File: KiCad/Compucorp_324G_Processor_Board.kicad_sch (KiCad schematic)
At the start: 9 parts, among them J5 Processor Interboard, J6 Unused Connector, U5 TMC1872 (TCL07), U6 TMC1866 (TCL06), U7 TMC1867 (TCL05), U8 TMC1870 (TCL04)

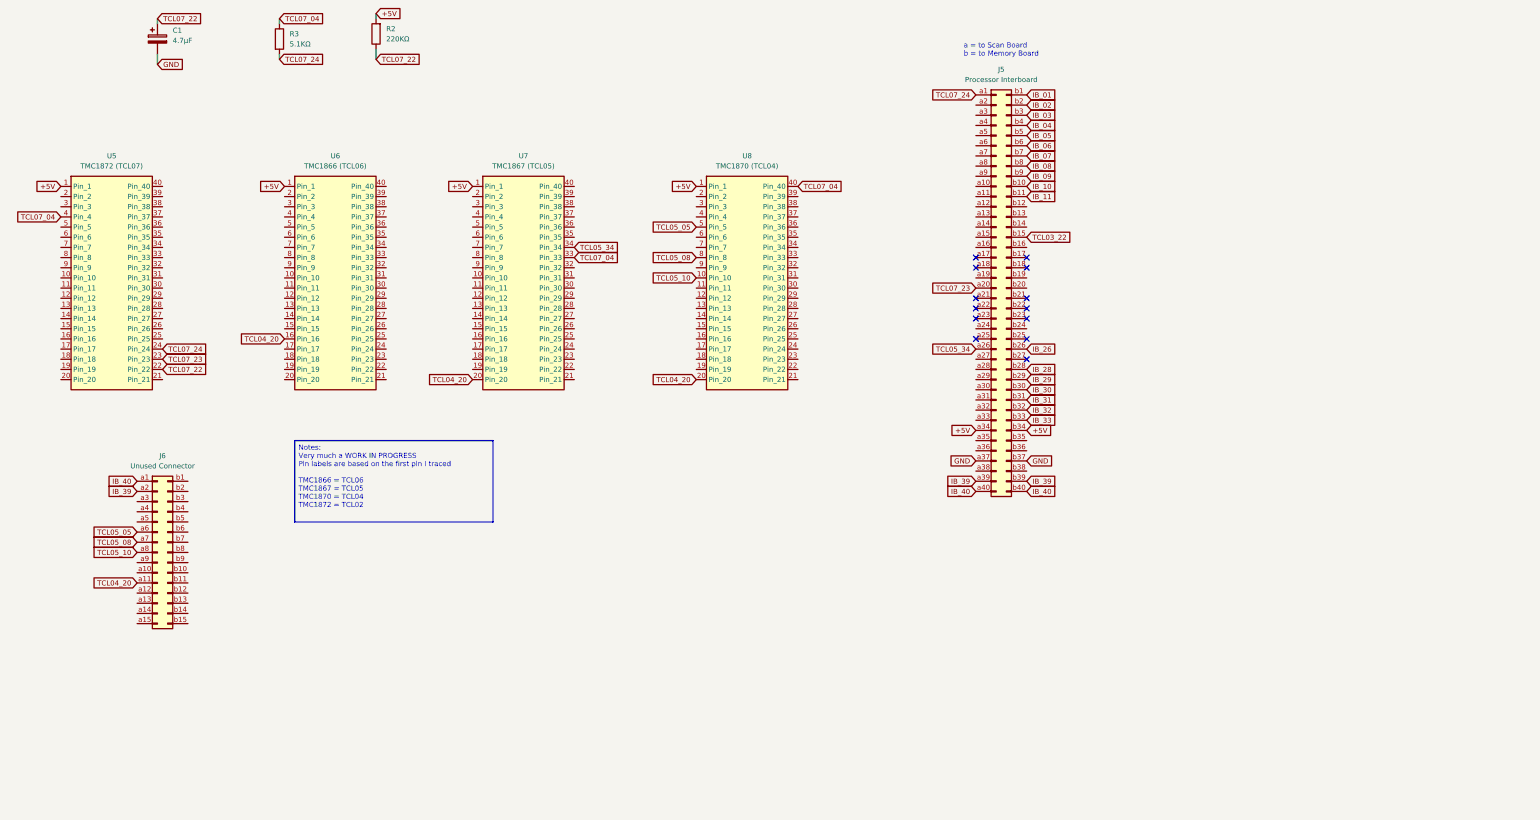
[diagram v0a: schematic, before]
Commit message: Update Compucorp_324G_Processor_Board.kicad_sch
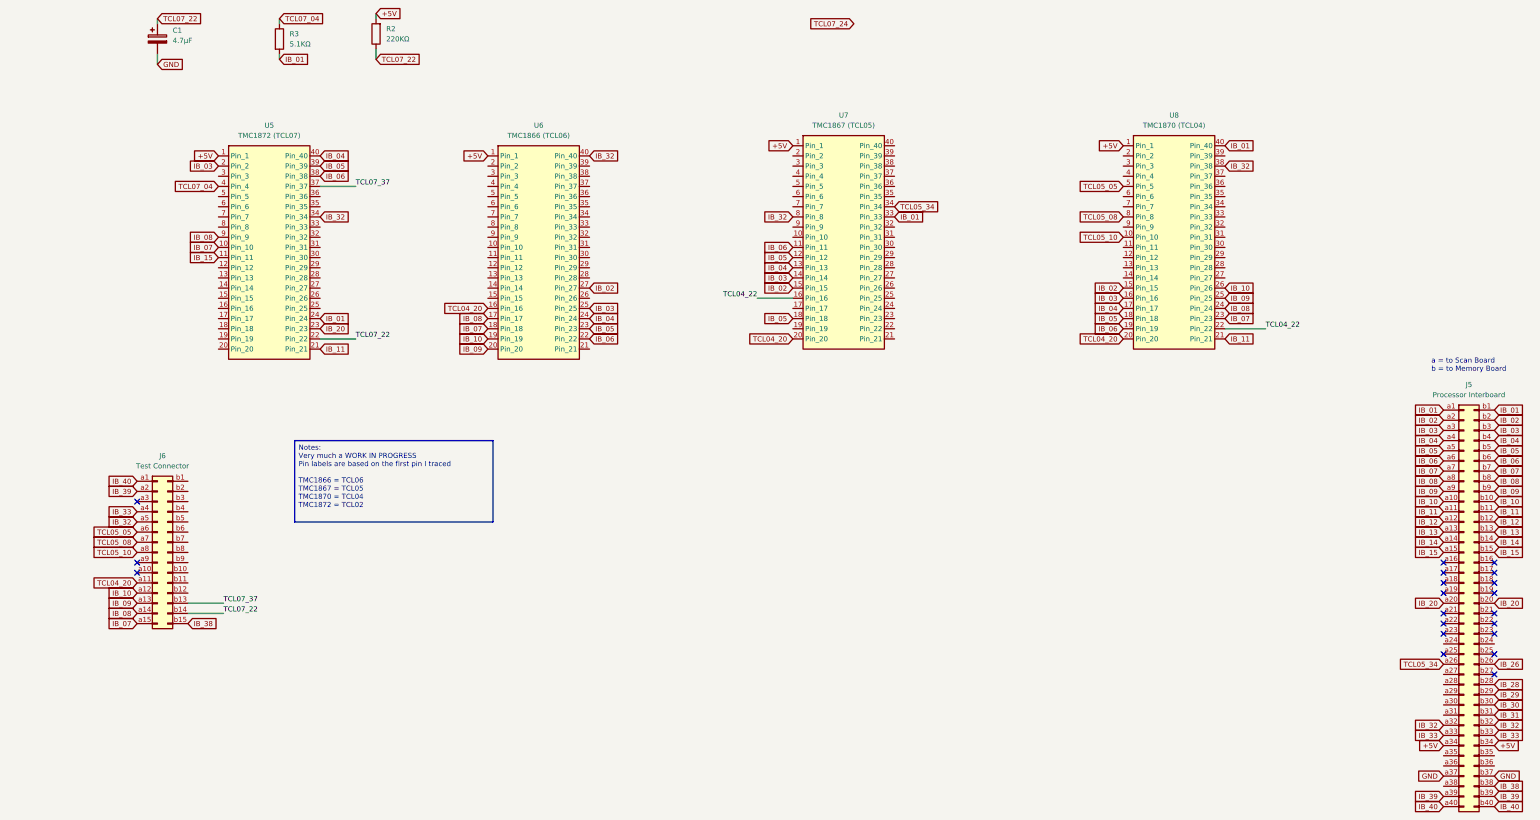
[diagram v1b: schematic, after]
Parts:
- J6: value Unused Connector -> Test Connector
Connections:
- net TCL03_22 is gone; now on net IB_15: J5.b15 (Pin_b15)
- net TCL07_23 is gone; now on net IB_20: J5.a20 (Pin_a20), U5.23 (Pin_23)
- net IB_01: now also J5.a1 (Pin_a1), R3.2, U5.24 (Pin_24), U7.33 (Pin_33), U8.40 (Pin_40)
- net IB_02: now also J5.a2 (Pin_a2), U6.27 (Pin_27), U7.15 (Pin_15), U8.15 (Pin_15)
- net IB_03: now also J5.a3 (Pin_a3), U5.2 (Pin_2), U6.25 (Pin_25), U7.14 (Pin_14), U8.16 (Pin_16)
- net IB_04: now also J5.a4 (Pin_a4), U5.40 (Pin_40), U6.24 (Pin_24), U7.13 (Pin_13), U8.17 (Pin_17)
- net IB_05: now also J5.a5 (Pin_a5), U5.39 (Pin_39), U6.23 (Pin_23), U7.12 (Pin_12), U7.18 (Pin_18), U8.18 (Pin_18)
- net IB_06: now also J5.a6 (Pin_a6), U5.38 (Pin_38), U6.22 (Pin_22), U7.11 (Pin_11), U8.19 (Pin_19)
- net IB_07: now also J5.a7 (Pin_a7), J6.a15 (Pin_a15), U5.10 (Pin_10), U6.18 (Pin_18), U8.23 (Pin_23)
- net IB_08: now also J5.a8 (Pin_a8), J6.a14 (Pin_a14), U5.9 (Pin_9), U6.17 (Pin_17), U8.24 (Pin_24)
- net IB_09: now also J5.a9 (Pin_a9), J6.a13 (Pin_a13), U6.20 (Pin_20), U8.25 (Pin_25)
- net IB_10: now also J5.a10 (Pin_a10), J6.a12 (Pin_a12), U6.19 (Pin_19), U8.26 (Pin_26)
- net IB_11: now also J5.a11 (Pin_a11), U5.21 (Pin_21), U8.21 (Pin_21)
- net IB_32: now also J5.a32 (Pin_a32), J6.a5 (Pin_a5), U5.34 (Pin_34), U6.40 (Pin_40), U7.8 (Pin_8), U8.38 (Pin_38)
- net IB_33: now also J5.a33 (Pin_a33), J6.a4 (Pin_a4)
- net TCL07_04: no longer U7.33 (Pin_33), U8.40 (Pin_40)
- net TCL07_22: now also J6.b14 (Pin_b14)
- net TCL07_24: no longer J5.a1 (Pin_a1), R3.2, U5.24 (Pin_24)
- net TCL04_22: now reaches U8.22 (Pin_22)
- net TCL04_22: now also U7.16 (Pin_16)
- net TCL07_37: now reaches J6.b13 (Pin_b13)
- net TCL07_37: now also U5.37 (Pin_37)
- net IB_38: now reaches J6.b15 (Pin_b15)
- net IB_38: now also J5.b38 (Pin_b38)
- net IB_15: now reaches U5.11 (Pin_11)
- net IB_15: now also J5.a15 (Pin_a15)
- net IB_12: now reaches J5.a12 (Pin_a12)
- net IB_12: now also J5.b12 (Pin_b12)
- net IB_13: now reaches J5.a13 (Pin_a13)
- net IB_13: now also J5.b13 (Pin_b13)
- net IB_14: now reaches J5.a14 (Pin_a14)
- net IB_14: now also J5.b14 (Pin_b14)
- net IB_20: now reaches J5.b20 (Pin_b20)
- no-connect marks 13 -> 20
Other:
- moved on the sheet: J5, U5, U6, U7, U8
